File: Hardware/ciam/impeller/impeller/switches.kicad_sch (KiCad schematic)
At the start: 61 parts, among them J10 Micro-Fit_2x3P, J7 Micro-Fit_2x5P, J8 Micro-Fit_2x5P, J9 Micro-Fit_2x2P, U10 TLP291, U11 TLP291, U12 TLP291, U13 TLP291, U14 TLP291, U15 TLP291, U16 TLP291, U17 TLP291, U18 TLP291, U21 TLP291, U22 TLP291, U23 TLP291, U24 TLP291, U25 TLP291, U4 B0505MT-1WR4, U9 TLP291

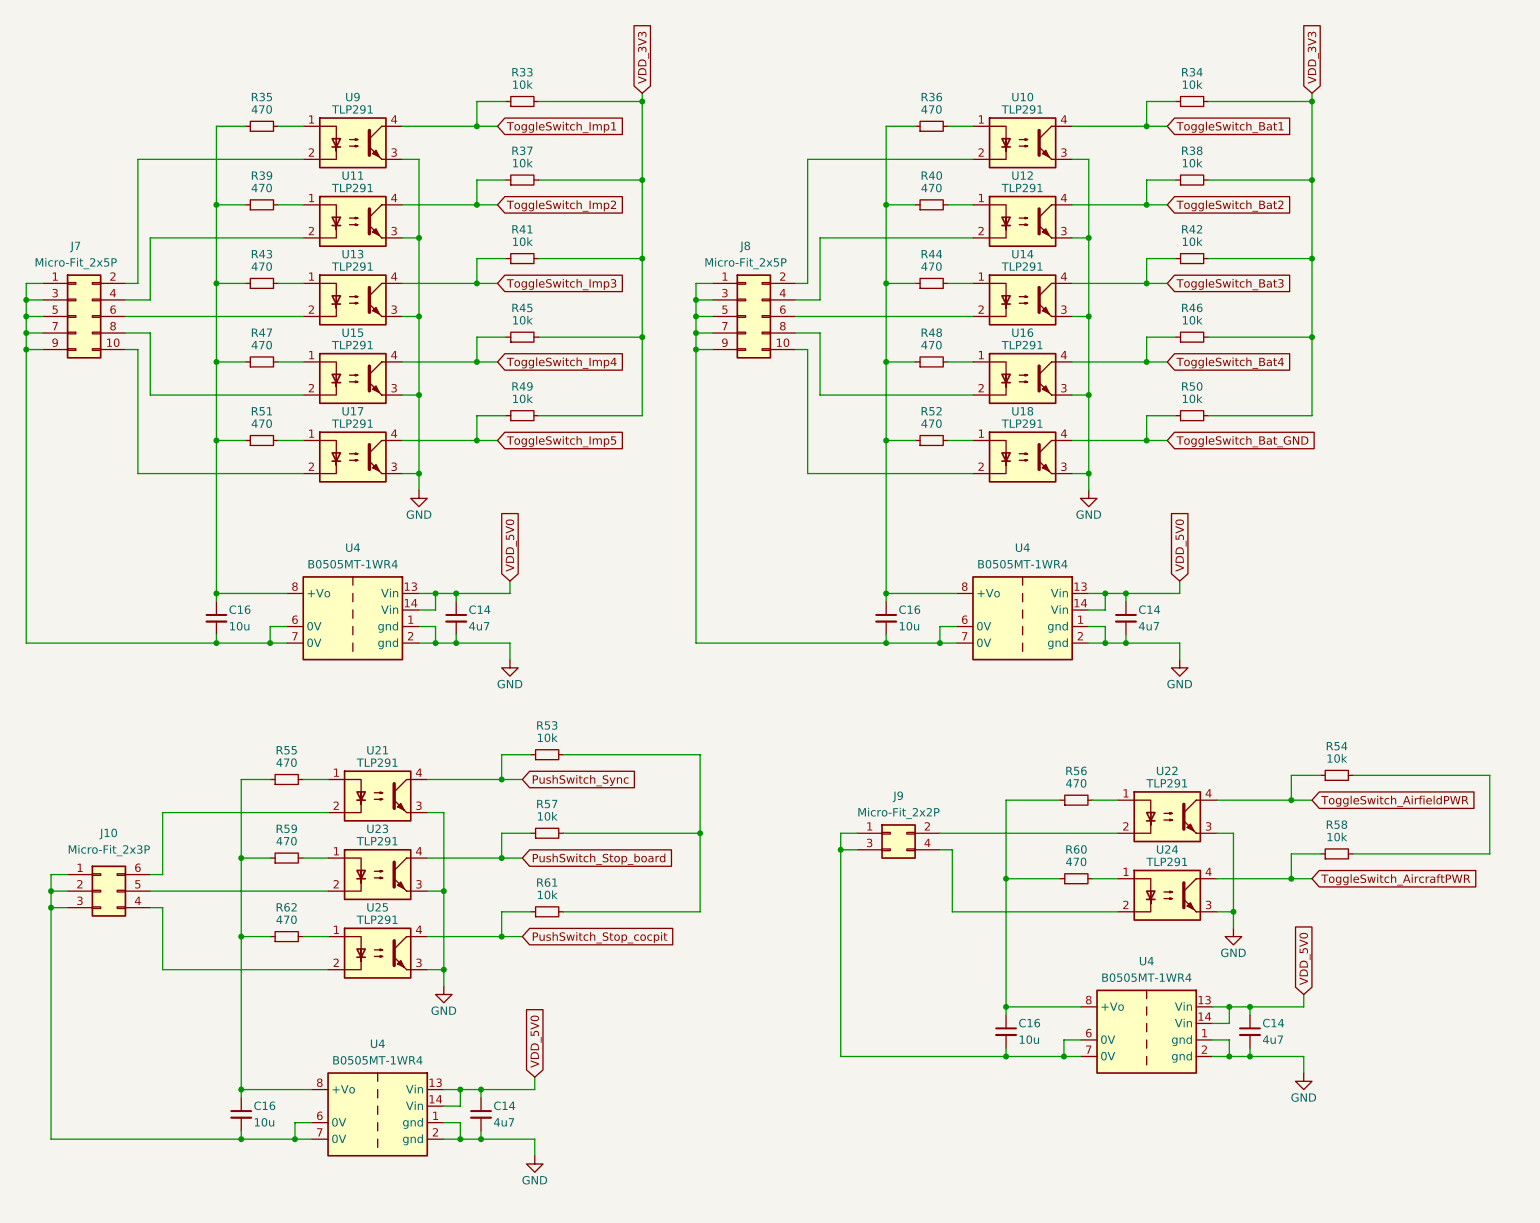
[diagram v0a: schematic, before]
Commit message: multiple fixes
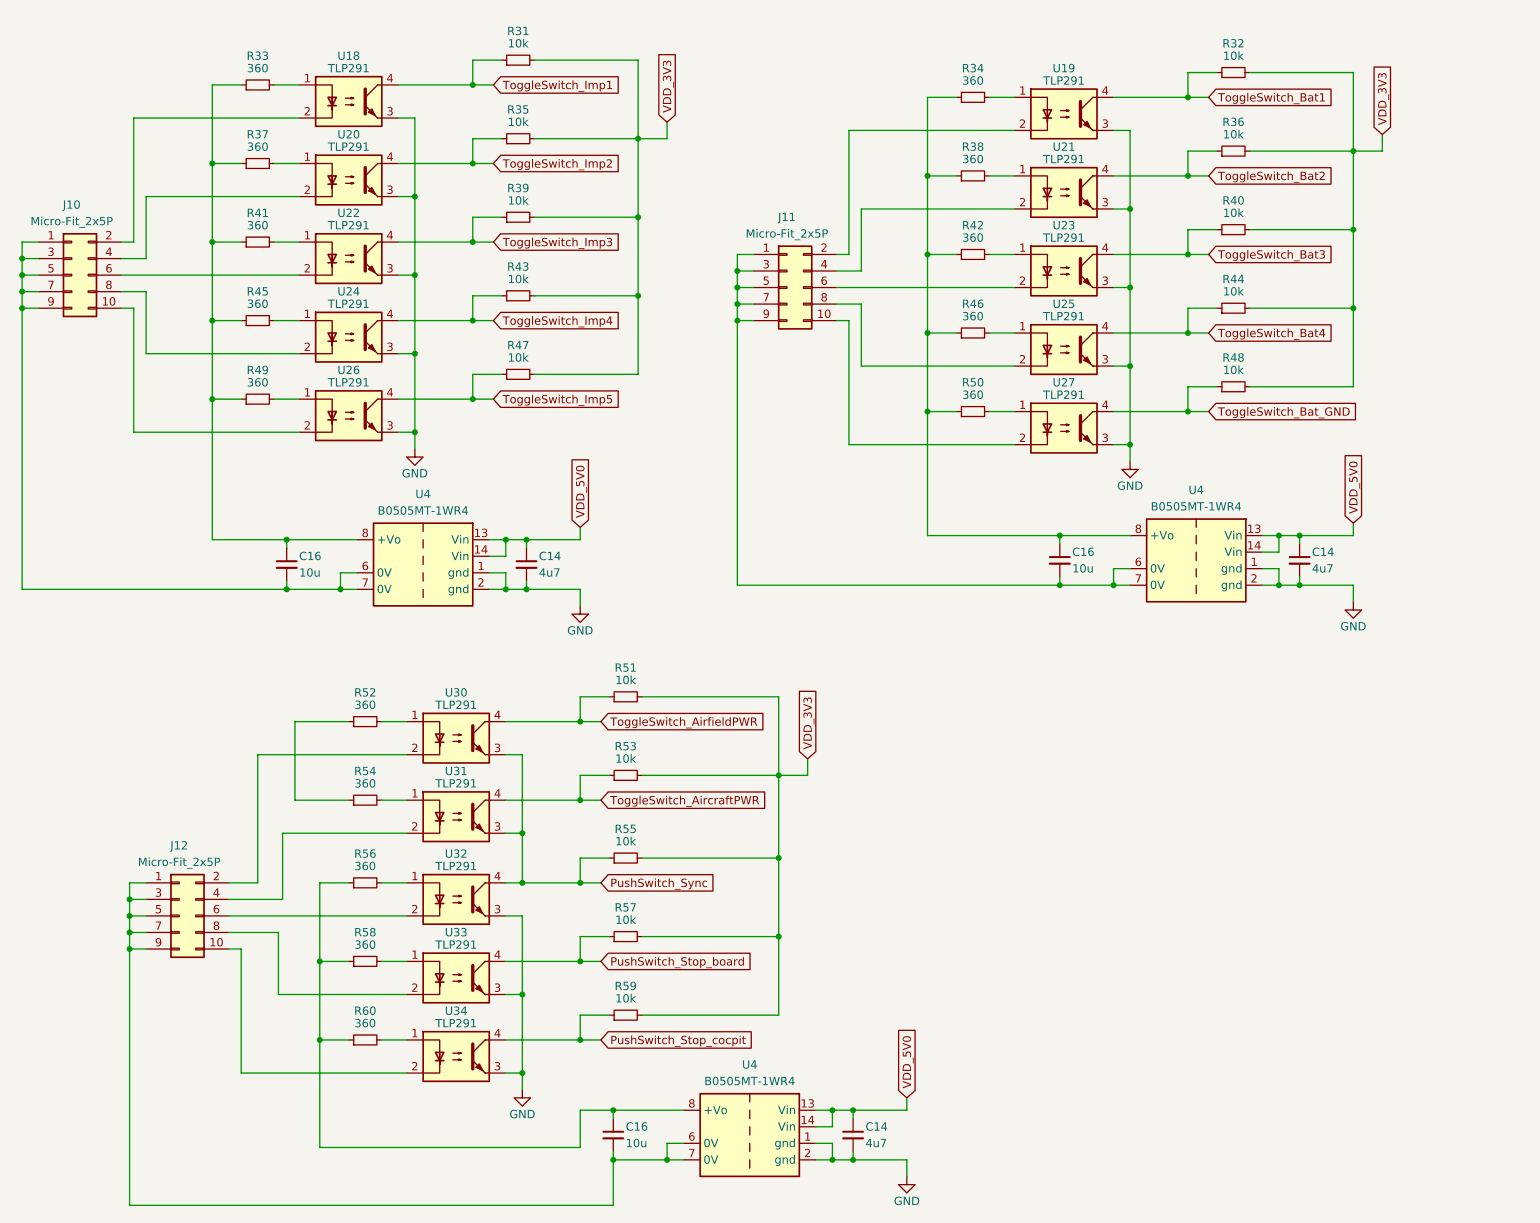
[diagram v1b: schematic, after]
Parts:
- removed C14: 4u7, symbol Device:C_Small
- removed C16: 10u, symbol Device:C_Small
- removed J10: Micro-Fit_2x3P, symbol Connector_Generic:Conn_02x03_Counter_Clockwise
- removed J9: Micro-Fit_2x2P, symbol Connector_Generic:Conn_02x02_Odd_Even
- removed R36, R39, R40, R43, R44, R47, R48, R51, R55, R59, R62: 470, symbol Device:R_Small
- removed U4: B0505MT-1WR4, symbol Interface_CAN_LIN:ISO1050DUB
- added J12: Micro-Fit_2x5P, symbol Connector_Generic:Conn_02x05_Odd_Even
- added R34, R37, R38, R41, R42, R45, R46, R49, R50, R54, R58: 360, Resistor_SMD:R_0603_1608Metric, symbol Device:R_Small
- C14: footprint (none) -> Capacitor_SMD:C_0805_2012Metric; Ссылка (none) -> https://www.chipdip.ru/product/grm21br61e475ka12l; Цена (none) -> 13
- C16: footprint (none) -> Capacitor_SMD:C_0805_2012Metric; Ссылка (none) -> https://www.chipdip.ru/product/grm21br61e106ka73l; Цена (none) -> 13
- J10: renamed from J7; Ссылка (none) -> https://www.chipdip.ru/product/sct3001fh-2x5p; Цена (none) -> 34
- J11: renamed from J8; Ссылка (none) -> https://www.chipdip.ru/product/sct3001fh-2x5p; Цена (none) -> 34
- R31: renamed from R33; footprint (none) -> Resistor_SMD:R_0805_2012Metric; Ссылка (none) -> https://www.chipdip.ru/product/0.125w-0805-10-kom-5; Цена (none) -> 5
- R32: renamed from R34; footprint (none) -> Resistor_SMD:R_0805_2012Metric; Ссылка (none) -> https://www.chipdip.ru/product/0.125w-0805-10-kom-5; Цена (none) -> 5
- R33: renamed from R35; value 470 -> 360; footprint (none) -> Resistor_SMD:R_0603_1608Metric; Ссылка (none) -> https://www.chipdip.ru/product/0.1w-0603-360-om-1; Цена (none) -> 5
- R35: renamed from R37; footprint (none) -> Resistor_SMD:R_0805_2012Metric; Ссылка (none) -> https://www.chipdip.ru/product/0.125w-0805-10-kom-5; Цена (none) -> 5
- R36: renamed from R38; footprint (none) -> Resistor_SMD:R_0805_2012Metric; Ссылка (none) -> https://www.chipdip.ru/product/0.125w-0805-10-kom-5; Цена (none) -> 5
- R39: renamed from R41; footprint (none) -> Resistor_SMD:R_0805_2012Metric; Ссылка (none) -> https://www.chipdip.ru/product/0.125w-0805-10-kom-5; Цена (none) -> 5
- R40: renamed from R42; footprint (none) -> Resistor_SMD:R_0805_2012Metric; Ссылка (none) -> https://www.chipdip.ru/product/0.125w-0805-10-kom-5; Цена (none) -> 5
- R43: renamed from R45; footprint (none) -> Resistor_SMD:R_0805_2012Metric; Ссылка (none) -> https://www.chipdip.ru/product/0.125w-0805-10-kom-5; Цена (none) -> 5
- R44: renamed from R46; footprint (none) -> Resistor_SMD:R_0805_2012Metric; Ссылка (none) -> https://www.chipdip.ru/product/0.125w-0805-10-kom-5; Цена (none) -> 5
- R47: renamed from R49; footprint (none) -> Resistor_SMD:R_0805_2012Metric; Ссылка (none) -> https://www.chipdip.ru/product/0.125w-0805-10-kom-5; Цена (none) -> 5
- R48: renamed from R50; footprint (none) -> Resistor_SMD:R_0805_2012Metric; Ссылка (none) -> https://www.chipdip.ru/product/0.125w-0805-10-kom-5; Цена (none) -> 5
- R51: renamed from R54; footprint (none) -> Resistor_SMD:R_0805_2012Metric; Ссылка (none) -> https://www.chipdip.ru/product/0.125w-0805-10-kom-5; Цена (none) -> 5
- R52, R56, R60: value 470 -> 360; footprint (none) -> Resistor_SMD:R_0603_1608Metric; Ссылка (none) -> https://www.chipdip.ru/product/0.1w-0603-360-om-1; Цена (none) -> 5
- R53: renamed from R58; footprint (none) -> Resistor_SMD:R_0805_2012Metric; Ссылка (none) -> https://www.chipdip.ru/product/0.125w-0805-10-kom-5; Цена (none) -> 5
- R55: renamed from R53; footprint (none) -> Resistor_SMD:R_0805_2012Metric; Ссылка (none) -> https://www.chipdip.ru/product/0.125w-0805-10-kom-5; Цена (none) -> 5
- R57: footprint (none) -> Resistor_SMD:R_0805_2012Metric; Ссылка (none) -> https://www.chipdip.ru/product/0.125w-0805-10-kom-5; Цена (none) -> 5
- R59: renamed from R61; footprint (none) -> Resistor_SMD:R_0805_2012Metric; Ссылка (none) -> https://www.chipdip.ru/product/0.125w-0805-10-kom-5; Цена (none) -> 5
- U18: renamed from U9; Ссылка (none) -> https://www.chipdip.ru/product/tlp291-gb-tp-se-t; Цена (none) -> 62
- U19: renamed from U10; Ссылка (none) -> https://www.chipdip.ru/product/tlp291-gb-tp-se-t; Цена (none) -> 62
- U20: renamed from U11; Ссылка (none) -> https://www.chipdip.ru/product/tlp291-gb-tp-se-t; Цена (none) -> 62
- U21: renamed from U12; Ссылка (none) -> https://www.chipdip.ru/product/tlp291-gb-tp-se-t; Цена (none) -> 62
- U22: renamed from U13; Ссылка (none) -> https://www.chipdip.ru/product/tlp291-gb-tp-se-t; Цена (none) -> 62
- U23: renamed from U14; Ссылка (none) -> https://www.chipdip.ru/product/tlp291-gb-tp-se-t; Цена (none) -> 62
- U24: renamed from U15; Ссылка (none) -> https://www.chipdip.ru/product/tlp291-gb-tp-se-t; Цена (none) -> 62
- U25: renamed from U16; Ссылка (none) -> https://www.chipdip.ru/product/tlp291-gb-tp-se-t; Цена (none) -> 62
- U26: renamed from U17; Ссылка (none) -> https://www.chipdip.ru/product/tlp291-gb-tp-se-t; Цена (none) -> 62
- U27: renamed from U18; Ссылка (none) -> https://www.chipdip.ru/product/tlp291-gb-tp-se-t; Цена (none) -> 62
- U30: renamed from U22; Ссылка (none) -> https://www.chipdip.ru/product/tlp291-gb-tp-se-t; Цена (none) -> 62
- U31: renamed from U24; Ссылка (none) -> https://www.chipdip.ru/product/tlp291-gb-tp-se-t; Цена (none) -> 62
- U32: renamed from U21; Ссылка (none) -> https://www.chipdip.ru/product/tlp291-gb-tp-se-t; Цена (none) -> 62
- U33: renamed from U23; Ссылка (none) -> https://www.chipdip.ru/product/tlp291-gb-tp-se-t; Цена (none) -> 62
- U34: renamed from U25; Ссылка (none) -> https://www.chipdip.ru/product/tlp291-gb-tp-se-t; Цена (none) -> 62
- U4: Ссылка (none) -> https://www.chipdip.ru/product0/8003333290; Цена (none) -> 120
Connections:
- net GND: no longer U30.3, U31.3
- net PushSwitch_Sync: now also U30.3, U31.3
- net VDD_3V3: now also R51.2, R53.2, R55.2, R57.2, R59.2
- net at U30.1: now also R52.2; no longer R56.2
- net at U30.2: now also J12.2 (Pin_2)
- net at U24.1: now also R45.2
- net at C16.1, U4.8 (+Vo): now also R56.1, R60.1, R58.1
- net at U34.1: now also R60.2
- net at C16.1, R33.1, U4.8 (+Vo): now also R37.1, R41.1, R45.1, R49.1
- net at U22.1: now also R41.2
- net at U34.2: now also J12.10 (Pin_10)
- net at C16.1, U4.8 (+Vo): now also R34.1, R38.1, R42.1, R46.1, R50.1; no longer R52.1
- net at U27.1: now also R50.2; no longer R52.2
- net at U33.1: now also R58.2
- net at U33.2: now also J12.8 (Pin_8)
- net at U19.1: now also R34.2
- net at U21.1: now also R38.2
- net at U31.1: now also R54.2; no longer R60.2
- net at C16.2, U4.6 (0V), U4.7 (0V): now also J12.1 (Pin_1), J12.3 (Pin_3), J12.5 (Pin_5), J12.7 (Pin_7), J12.9 (Pin_9)
- net at U32.2: now also J12.6 (Pin_6)
- net at U25.1: now also R46.2
- net at U26.1: now also R49.2
- net at U23.1: now also R42.2
- net at U32.1: now also R56.2
- net at U20.1: now also R37.2
- net at U31.2: now also J12.4 (Pin_4)
- new net: R52.1, R54.1
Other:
- moved on the sheet: C14, C16, J10, J11, R31, R32, R33, R35, R36, R39, R40, R43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

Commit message: updated bom
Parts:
- C14: Человекопонятное название (none) -> Конденсатор 4.7мкФ
- C16: Человекопонятное название (none) -> Конденсатор 10мкФ
- J10, J11, J12: Человекопонятное название (none) -> Разъем Micro-Fit 2x5 М
- R31, R32, R35, R36, R39, R40, R43, R44, R47, R48, R51, R53, R55, R57, R59: Человекопонятное название (none) -> Резистор 10k Ом
- R33, R34, R37, R38, R41, R42, R45, R46, R49, R50, R52, R54, R56, R58, R60: Человекопонятное название (none) -> Резистор 360 Ом
- U18, U19, U20, U21, U22, U23, U24, U25, U26, U27, U30, U31, U32, U33, U34: Человекопонятное название (none) -> Оптопара с транзисторным выходом
- U4: Человекопонятное название (none) -> DC/DC преобразователь
